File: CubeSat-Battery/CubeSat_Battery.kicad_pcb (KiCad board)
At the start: 2 copper layers, 92 x 92 mm, 5 parts, among them J1 Conn_01x02_Pin, J2 Conn_01x02_Pin, U1 BatteryPack

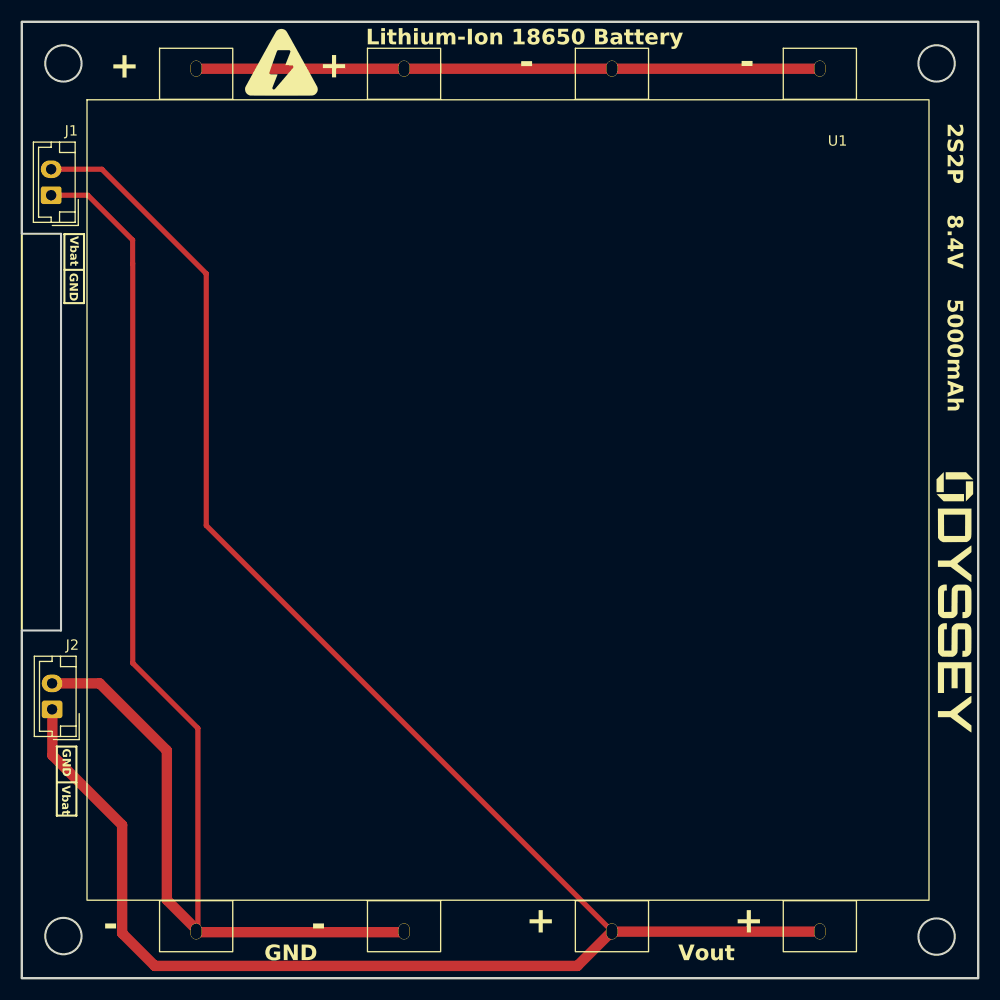
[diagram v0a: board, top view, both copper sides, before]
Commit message: Mostly fine tuning the boards, also added capacitor for battery ADC
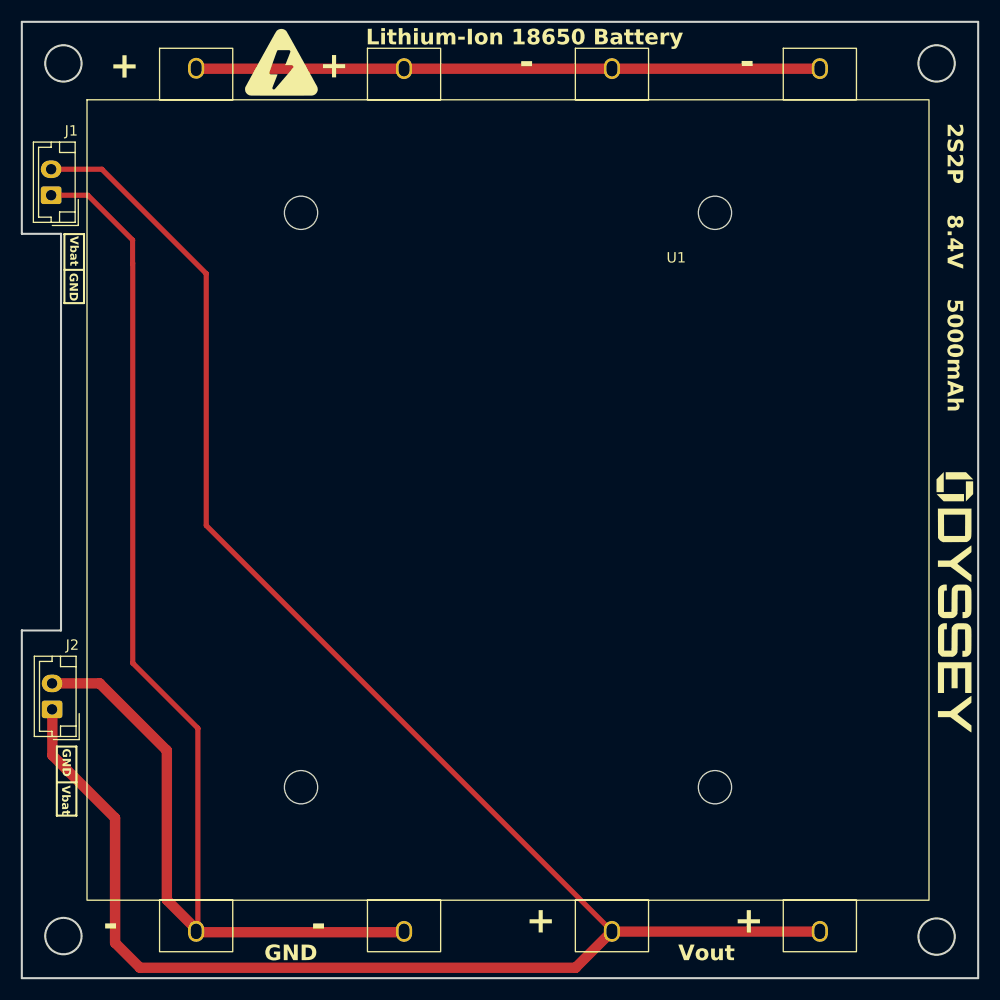
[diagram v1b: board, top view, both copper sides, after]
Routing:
- net Vbat_8.4V: track 192.3 -> 193.3 mm
